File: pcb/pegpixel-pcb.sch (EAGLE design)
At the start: 15 parts

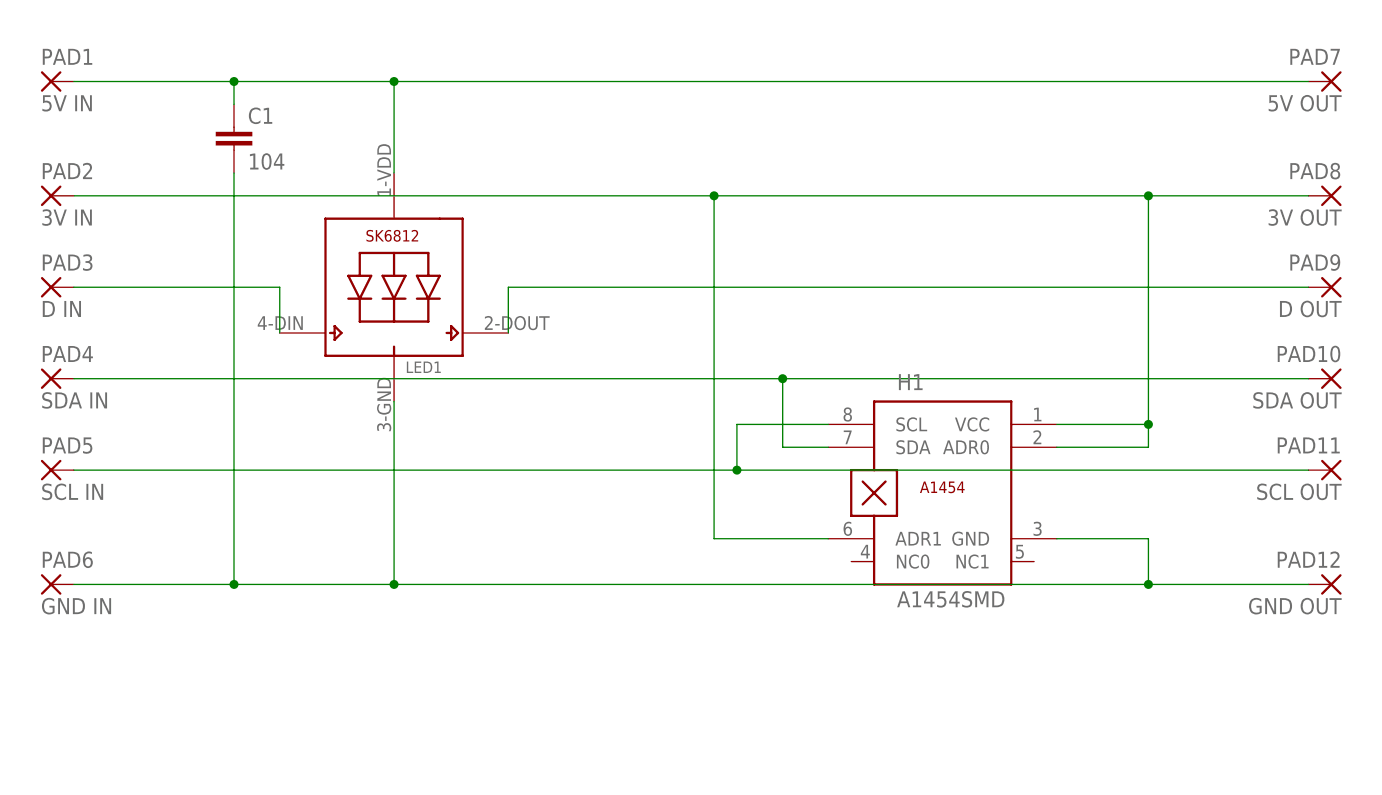
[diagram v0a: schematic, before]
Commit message: add first pcb layout
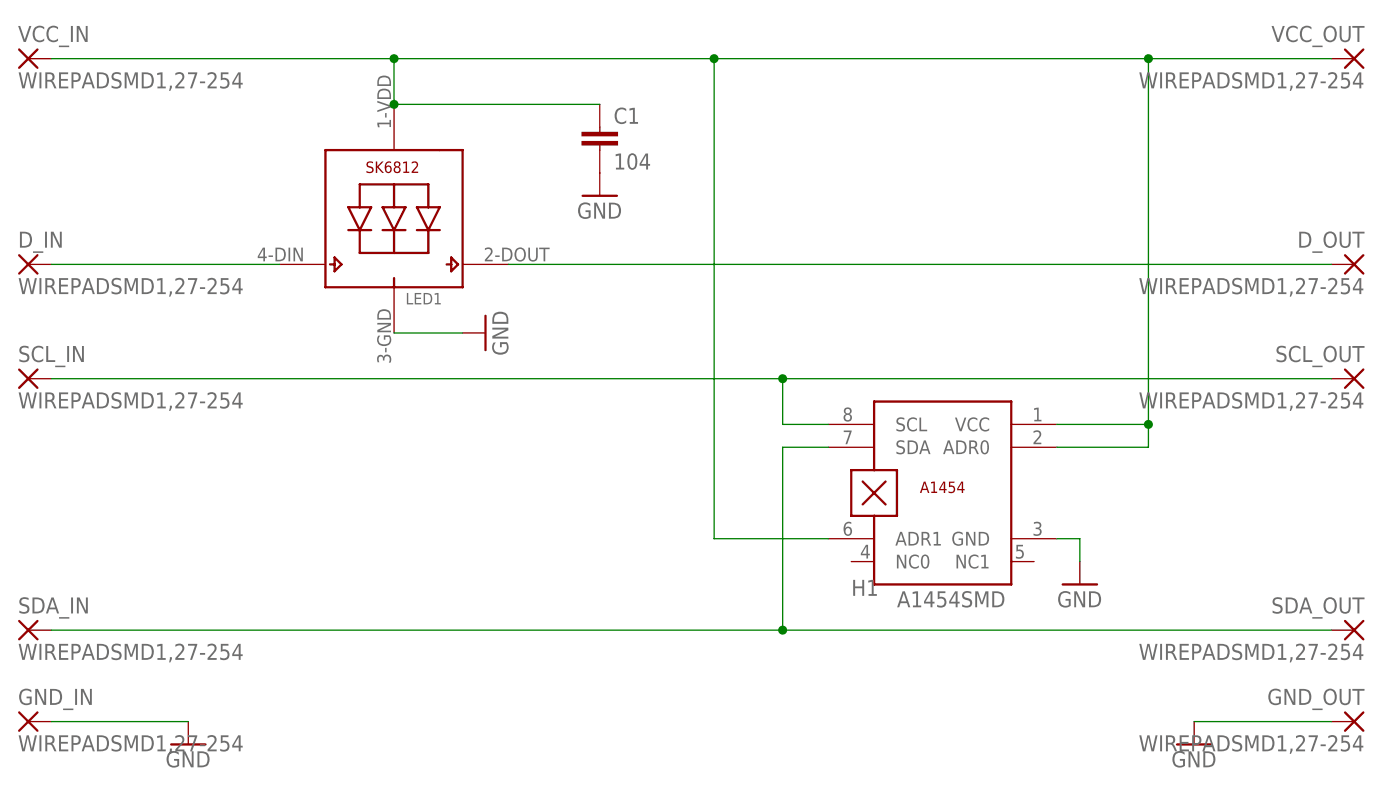
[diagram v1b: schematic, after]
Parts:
- removed PAD1: 5V IN, wirepad:1,6/0,8
- removed PAD10: SDA OUT, wirepad:1,6/0,8
- removed PAD11: SCL OUT, wirepad:1,6/0,8
- removed PAD12: GND OUT, wirepad:1,6/0,8
- removed PAD2: 3V IN, wirepad:1,6/0,8
- removed PAD3: D IN, wirepad:1,6/0,8
- removed PAD4: SDA IN, wirepad:1,6/0,8
- removed PAD5: SCL IN, wirepad:1,6/0,8
- removed PAD6: GND IN, wirepad:1,6/0,8
- removed PAD7: 5V OUT, wirepad:1,6/0,8
- removed PAD8: 3V OUT, wirepad:1,6/0,8
- removed PAD9: D OUT, wirepad:1,6/0,8
- added D_IN, D_OUT, GND_IN, GND_OUT, SCL_IN, SCL_OUT, SDA_IN, SDA_OUT, VCC_IN, VCC_OUT: WIREPADSMD1,27-254, wirepad:WIREPADSMD1,27-254
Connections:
- removed net N$1: C1.1, LED1.VDD, PAD1.P, PAD7.P
- removed net N$3: C1.2, H1.GND, LED1.GND, PAD12.P, PAD6.P
- new net GND: C1.2, GND_IN.P, GND_OUT.P, H1.GND, LED1.GND
- net N$2: now also C1.1, LED1.VDD, VCC_IN.P, VCC_OUT.P; no longer PAD2.P, PAD8.P
- net N$4: now also SCL_IN.P, SCL_OUT.P; no longer PAD11.P, PAD5.P
- net N$5: now also SDA_IN.P, SDA_OUT.P; no longer PAD10.P, PAD4.P
- net N$6: now also D_IN.P; no longer PAD3.P
- net N$7: now also D_OUT.P; no longer PAD9.P
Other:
- moved on the sheet: C1, LED1
